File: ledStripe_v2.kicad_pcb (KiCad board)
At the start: 2 copper layers, 122.4 x 6.1 mm, 16 parts, among them J101 Conn_01x03

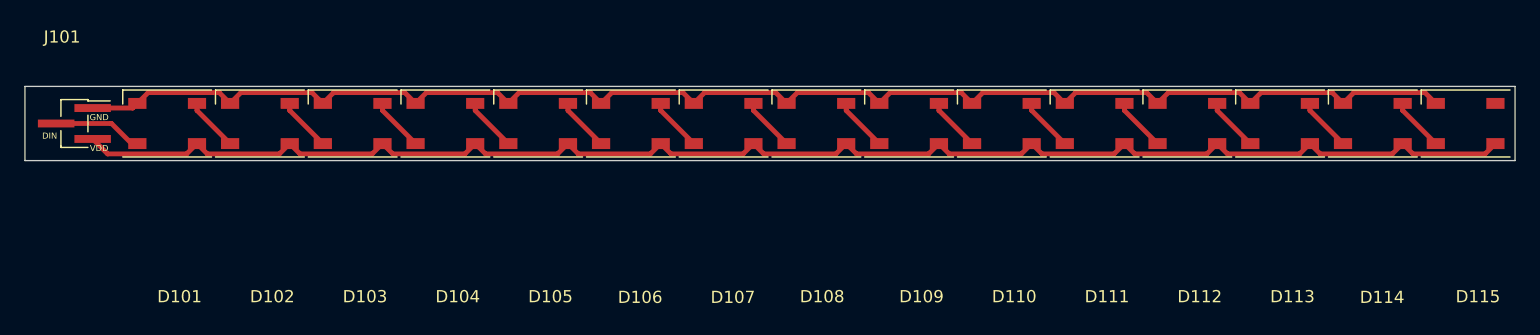
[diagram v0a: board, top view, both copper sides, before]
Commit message: final version
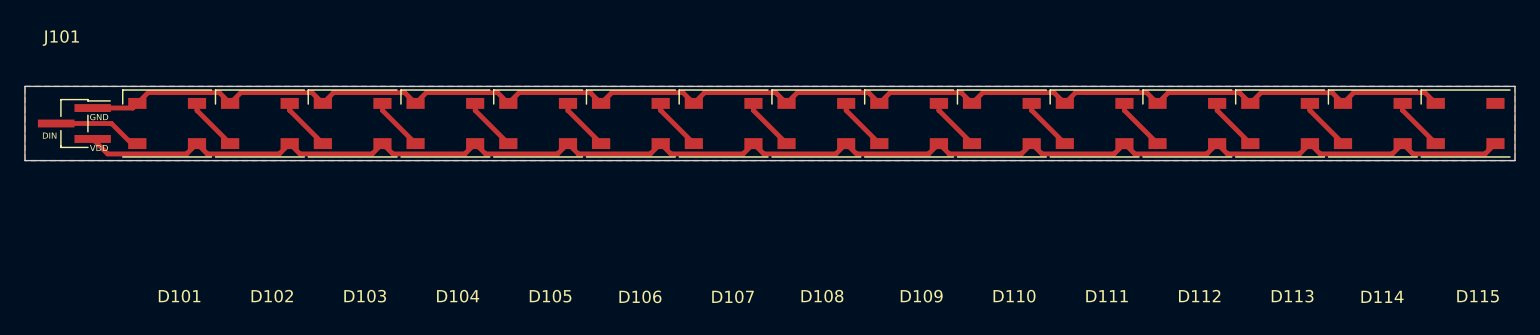
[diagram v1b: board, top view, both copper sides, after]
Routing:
- added copper zone on B.Cu, net (none)
- added copper zone on F.Cu, net (none)
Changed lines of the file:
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@@
       (outputformat 1)
       (mirror false)
-      (drillshape 1)
+      (drillshape 0)
       (scaleselection 1)
-      (outputdirectory "")
+      (outputdirectory "gerber/")
     )
   )
@@
   (segment (start 190.59 88.01) (end 187.87 85.29) (width 0.4) (layer "F.Cu") (net 17))
   (segment (start 187.87 85.29) (end 187.87 84.71) (width 0.4) (layer "F.Cu") (net 17))
+  (zone (net 0) (net_name "") (layer "F.Cu") (hatch edge 0.508)
+    (connect_pads (clearance 0.508))
+    (min_thickness 0.254) (filled_areas_thickness no)
+    (fill yes (thermal_gap 0.508) (thermal_bridge_width 0.508))
+    (polygon
+      (pts
+        (xy 204.724 89.408)
+        (xy 82.296 89.408)
+        (xy 82.296 83.312)
+        (xy 204.724 83.312)
+      )
+    )
+  )
+  (zone (net 0) (net_name "") (layer "B.Cu") (hatch edge 0.508)
+    (connect_pads (clearance 0.508))
+    (min_thickness 0.254) (filled_areas_thickness no)
+    (fill yes (thermal_gap 0.508) (thermal_bridge_width 0.508))
+    (polygon
+      (pts
+        (xy 204.724 89.408)
+        (xy 82.296 89.408)
+        (xy 82.296 83.312)
+        (xy 204.724 83.312)
+      )
+    )
+  )
 )
